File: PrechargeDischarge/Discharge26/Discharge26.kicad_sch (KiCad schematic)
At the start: 7 parts, among them J1 HV_Conn, J2 LV_Conn, K4 Relay_SPST-NC, Q1 Q_NMOS_GSD

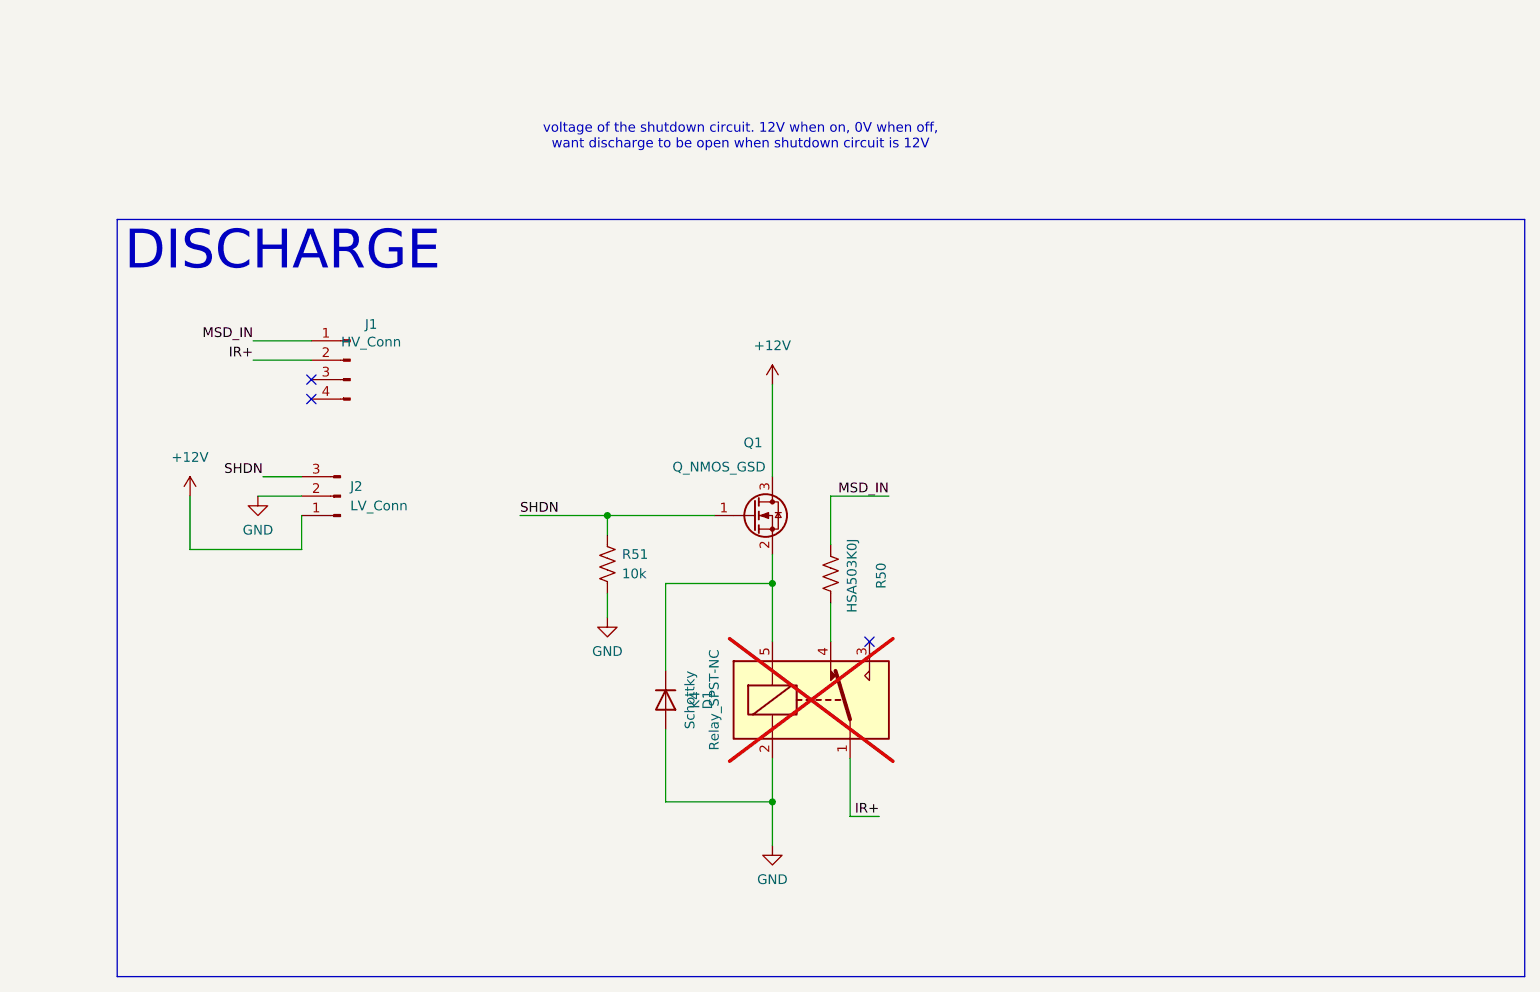
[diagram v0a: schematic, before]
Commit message: Discharge
guys its gonns work this time
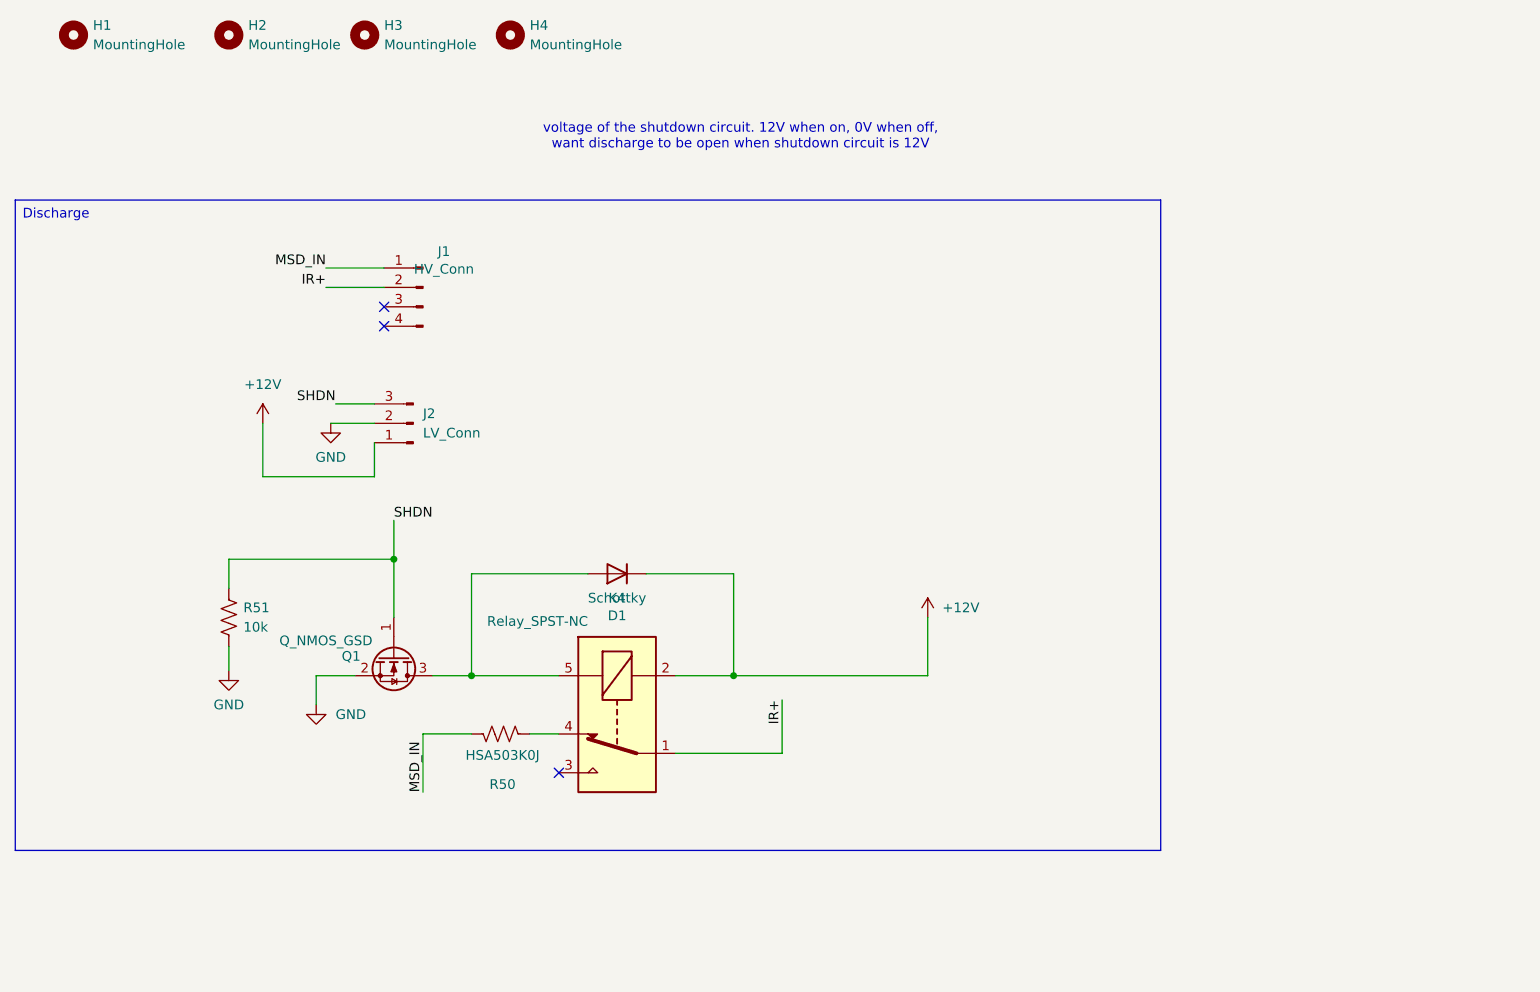
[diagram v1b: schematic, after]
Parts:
- added H1, H2, H3, H4: MountingHole, MountingHole:MountingHole_2.2mm_M2, symbol Mechanical:MountingHole
- K4: now fitted
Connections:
- net +12V: now also D1.1 (K), K4.2; no longer Q1.3 (D)
- net GND: now also Q1.2 (S); no longer D1.2 (A), K4.2
- new net: D1.2 (A), K4.5, Q1.3 (D)
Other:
- moved on the sheet: D1, J1, J2, Q1, R50, R51
